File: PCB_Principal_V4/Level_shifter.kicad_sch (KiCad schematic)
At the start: 3 parts, among them Q4 SI2302S

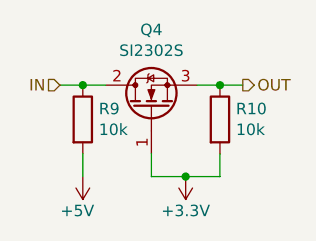
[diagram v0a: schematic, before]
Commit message: update
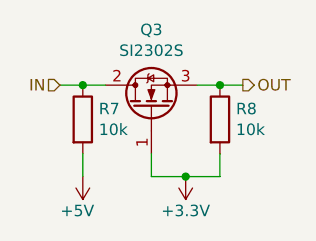
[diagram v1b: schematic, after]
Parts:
- renumbered Q4 to Q3, R9 to R7, R10 to R8
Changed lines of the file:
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@@
   (symbol (lib_id "Device:Q_NMOS_GDS") (at 74.93 40.64 90)
     (in_bom yes) (on_board yes)
-    (property "Reference" "Q4" (id 0) (at 74.93 31.9532 90))
+    (property "Reference" "Q3" (id 0) (at 74.93 31.9532 90))
     (property "Value" "SI2302S" (id 1) (at 74.93 34.2646 90))
     (property "Footprint" "Package_TO_SOT_SMD:SOT-23" (id 2) (at 72.39 35.56 0)
@@
   (symbol (lib_id "Device:R") (at 67.31 41.91 0)
     (in_bom yes) (on_board yes)
-    (property "Reference" "R9" (id 0) (at 69.088 40.7416 0)
+    (property "Reference" "R7" (id 0) (at 69.088 40.7416 0)
       (effects (font (size 1.27 1.27)) (justify left))
     )
@@
   (symbol (lib_id "power:+5V") (at 67.31 48.26 180)
     (in_bom yes) (on_board yes)
-    (property "Reference" "#PWR0144" (id 0) (at 67.31 44.45 0)
+    (property "Reference" "#PWR0142" (id 0) (at 67.31 44.45 0)
       (effects (font (size 1.27 1.27)) hide)
     )
@@
   (symbol (lib_id "Device:R") (at 82.55 41.91 0)
     (in_bom yes) (on_board yes)
-    (property "Reference" "R10" (id 0) (at 84.328 40.7416 0)
+    (property "Reference" "R8" (id 0) (at 84.328 40.7416 0)
       (effects (font (size 1.27 1.27)) (justify left))
     )
@@
   (symbol (lib_id "power:+3.3V") (at 78.74 48.26 180)
     (in_bom yes) (on_board yes)
-    (property "Reference" "#PWR0143" (id 0) (at 78.74 44.45 0)
+    (property "Reference" "#PWR0141" (id 0) (at 78.74 44.45 0)
       (effects (font (size 1.27 1.27)) hide)
     )

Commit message: update last PCBs
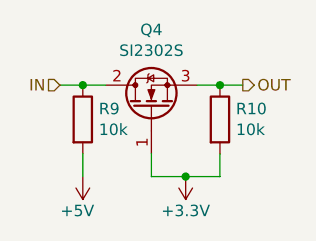
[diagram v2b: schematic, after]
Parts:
- renumbered Q3 to Q4, R8 to R10, R7 to R9
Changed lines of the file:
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@@
   (symbol (lib_id "Device:Q_NMOS_GDS") (at 74.93 40.64 90)
     (in_bom yes) (on_board yes)
-    (property "Reference" "Q3" (id 0) (at 74.93 31.9532 90))
+    (property "Reference" "Q4" (id 0) (at 74.93 31.9532 90))
     (property "Value" "SI2302S" (id 1) (at 74.93 34.2646 90))
     (property "Footprint" "Package_TO_SOT_SMD:SOT-23" (id 2) (at 72.39 35.56 0)
@@
   (symbol (lib_id "Device:R") (at 67.31 41.91 0)
     (in_bom yes) (on_board yes)
-    (property "Reference" "R7" (id 0) (at 69.088 40.7416 0)
+    (property "Reference" "R9" (id 0) (at 69.088 40.7416 0)
       (effects (font (size 1.27 1.27)) (justify left))
     )
@@
   (symbol (lib_id "power:+5V") (at 67.31 48.26 180)
     (in_bom yes) (on_board yes)
-    (property "Reference" "#PWR0142" (id 0) (at 67.31 44.45 0)
+    (property "Reference" "#PWR0144" (id 0) (at 67.31 44.45 0)
       (effects (font (size 1.27 1.27)) hide)
     )
@@
   (symbol (lib_id "Device:R") (at 82.55 41.91 0)
     (in_bom yes) (on_board yes)
-    (property "Reference" "R8" (id 0) (at 84.328 40.7416 0)
+    (property "Reference" "R10" (id 0) (at 84.328 40.7416 0)
       (effects (font (size 1.27 1.27)) (justify left))
     )
@@
   (symbol (lib_id "power:+3.3V") (at 78.74 48.26 180)
     (in_bom yes) (on_board yes)
-    (property "Reference" "#PWR0141" (id 0) (at 78.74 44.45 0)
+    (property "Reference" "#PWR0143" (id 0) (at 78.74 44.45 0)
       (effects (font (size 1.27 1.27)) hide)
     )
